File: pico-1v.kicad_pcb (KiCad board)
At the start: 4 copper layers, 54 x 26 mm, 44 parts, among them J2 USB-C-2.0, J3 Header-1, J4 Header-2, J5 SWD, SW1 UK-B0273-SP25Y, SW2 USB Boot, SW4 SW_Slide_DPDT, U1 RP2040, U2 MCP1703Ax-180xxTT, U3 MCP1703Ax-330xxTT, U4 AT25FF161A-SSHN-T, Y1 ECS-3225MV-120-BN-TR3

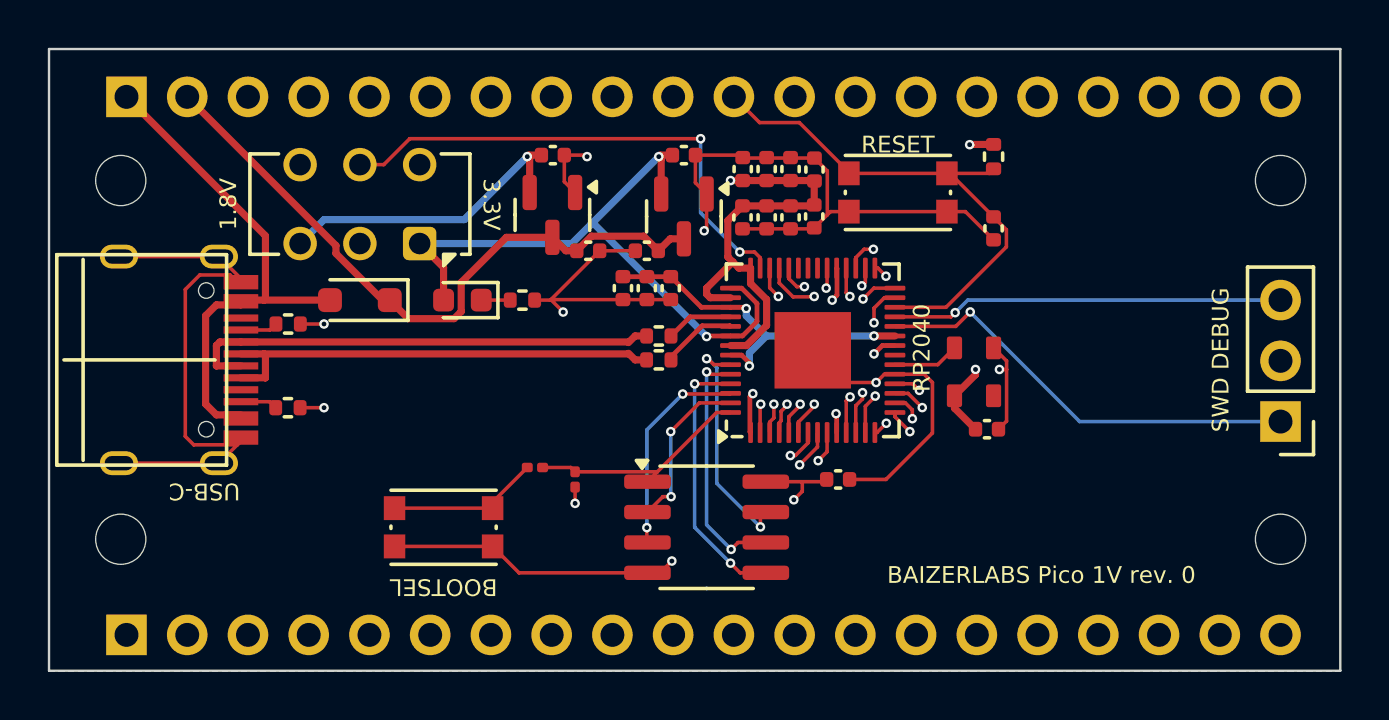
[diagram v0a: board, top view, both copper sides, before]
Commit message: Various fixes
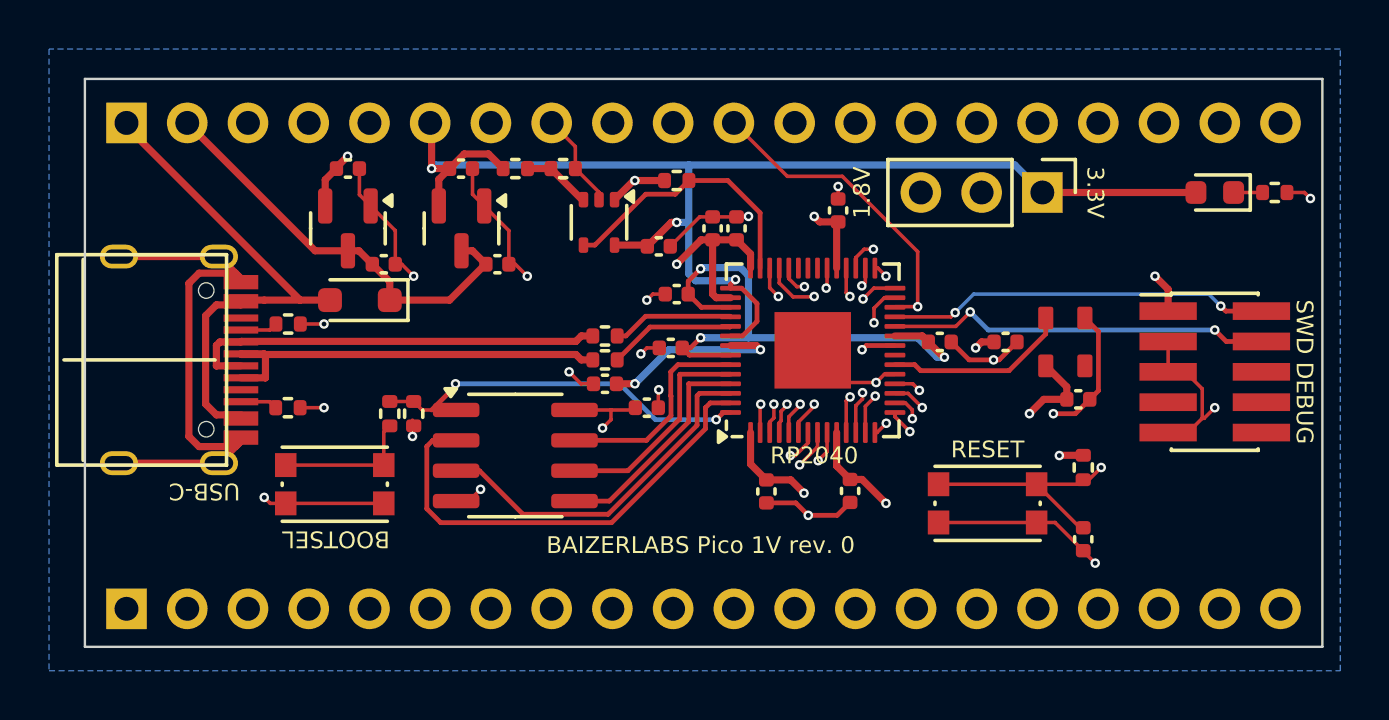
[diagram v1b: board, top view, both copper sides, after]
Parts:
- removed C12: 0.1uF, Capacitor_SMD:C_0402_1005Metric
- removed H1, H2, H3, H4: MountingHole, MountingHole:MountingHole_2.1mm
- removed SW4: SW_Slide_DPDT, Button_Switch_THT:SW_CK_JS202011CQN_DPDT_Straight
- added C18: C, Capacitor_SMD:C_0402_1005Metric, F.Cu at (147.5, 91.2)
- added J2: VOLTSEL, Connector_PinHeader_2.54mm:PinHeader_1x03_P2.54mm_Vertical, F.Cu at (163.5, 89.0)
- added R10: 10k, Resistor_SMD:R_0402_1005Metric, F.Cu at (143.5, 88.0)
- added R11: 10k, Resistor_SMD:R_0402_1005Metric, F.Cu at (148.2, 88.5)
- added R9: 1k, Resistor_SMD:R_0402_1005Metric, F.Cu at (141.5, 88.0)
- added U5: LMV331, Package_TO_SOT_SMD:SOT-353_SC-70-5, F.Cu at (145.0, 90.2)
- C1, C17: value 100n -> 0.1uF
- C13, C14, C15, C16: value 10u -> 10uF
- J5: value SWD -> Conn_02x05_Odd_Even; footprint Connector_PinHeader_2.54mm:PinHeader_1x03_P2.54mm_Vertical -> Connector_PinHeader_1.27mm:PinHeader_2x05_P1.27mm_Vertical_SMD
- R1, R2: footprint Resistor_SMD:R_0201_0603Metric -> Resistor_SMD:R_0402_1005Metric
- moved D3 31.8 mm to (170.8, 89.0)
- moved R7 31.8 mm to (173.3, 89.0)
- moved C9 14.2 mm to (155.5, 101.5), turned to -90 degrees
- moved C19 13.5 mm to (165.2, 103.5)
- moved R8 13.5 mm to (165.2, 100.5)
- moved SW1 13.5 mm to (161.2, 102.0)
- moved C10 13.5 mm to (152.0, 101.5), turned to -90 degrees
- moved C4 13.4 mm to (159.2, 95.2), turned to 0 degrees
- moved C11 11.9 mm to (145.2, 97.0), turned to 180 degrees
- moved C13 11.0 mm to (136.0, 92.0), turned to 0 degrees
- moved C8 9.57 mm to (162.0, 95.2), turned to 0 degrees
- moved C16 9.34 mm to (139.2, 88.0)
- moved U3 9.31 mm to (139.2, 90.5)
- moved C14 8.59 mm to (134.5, 88.0)
- moved U2 8.57 mm to (134.5, 90.5)
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- renumbered J2 to J1, R8 to R7, R9 to R8
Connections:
- net Net-(U1-USB_DM) renamed /USB_DM
- net Net-(U1-USB_DP) renamed /USB_DP
- J4 pad 4: /V_EN -> unconnected-(J4-Pin_4-Pad4)
- J4 pad 6: /AREF -> +3V3
- J5 pad 1: SWCLK -> VDD
- J5 pad 2: GND -> SWDIO
- J5 pad 3: SWDIO -> GND
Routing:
- net +3V3: track 27.6 -> 53.8 mm, vias 2 -> 3
- net VDD: track 31.8 -> 46.7 mm, vias 9 -> 14
- net +1V8: track 13.2 -> 27.1 mm
- net QSPI_SD1: track 6.98 -> 19.5 mm, vias 2 -> 0
- net RUN: track 22.2 -> 33.9 mm, vias 0 -> 2
- net VOLTAGE_MODE: track 21.5 -> 11.4 mm, vias 2 -> 0
- net VSYS: track 27.9 -> 17.9 mm
- net +1V1: track 15.2 -> 24.1 mm
- net QSPI_SS: track 9.55 -> 16.7 mm, vias 0 -> 2
- net QSPI_SD2: track 8.85 -> 15.0 mm, vias 2 -> 0
- net XIN: track 2.78 -> 7.71 mm
- net GND: track 88.7 -> 85.8 mm, vias 8 -> 19
- net Net-(U5--): track 0.00 -> 2.88 mm
- net GPIO2: track 27.3 -> 24.9 mm
- net /USB_DM: track 2.82 -> 5.09 mm
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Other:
- board size 54 x 26 mm -> 51.8 x 23.8 mm
